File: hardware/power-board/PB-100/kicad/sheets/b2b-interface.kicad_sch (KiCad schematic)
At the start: 1 part

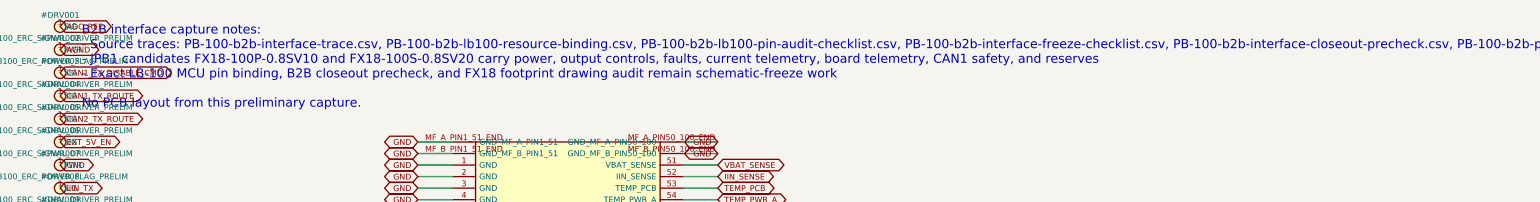
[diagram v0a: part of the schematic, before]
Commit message: feat(hardware): close LB FB schematics and FX18 mechanics
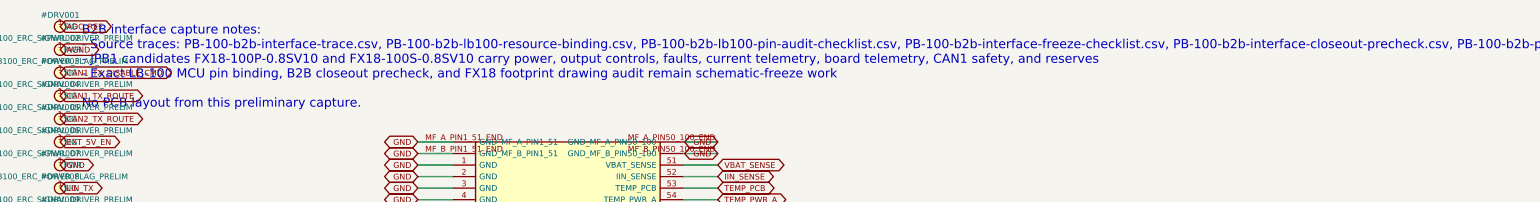
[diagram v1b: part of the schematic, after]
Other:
- note added: "B2B interface capture notes: - Source traces: PB-100-b2b-interface-trace.csv, PB-100-b2b-lb100-resource-binding.csv, PB-100-b2b-lb100-pin-audit-checklist.csv, PB-100-b2b-interface-freeze-checklist.csv, PB-100-b2b-interface-closeout-precheck.csv, PB-100-b2b-pin-map.csv, PB-100-b2b-pin-budget.csv - JPB1 candidates FX18-100P-0.8SV10 and FX18-100S-0.8SV10 carry power, output controls, faults, current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"
- note removed: "B2B interface capture notes: - Source traces: PB-100-b2b-interface-trace.csv, PB-100-b2b-lb100-resource-binding.csv, PB-100-b2b-lb100-pin-audit-checklist.csv, PB-100-b2b-interface-freeze-checklist.csv, PB-100-b2b-interface-closeout-precheck.csv, PB-100-b2b-pin-map.csv, PB-100-b2b-pin-budget.csv - JPB1 candidates FX18-100P-0.8SV10 and FX18-100S-0.8SV20 carry power, output controls, faults, current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"
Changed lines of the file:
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@@
     (comment 2 "Sources: PB-100-b2b-interface-trace.csv, PB-100-b2b-lb100-resource-binding.csv, PB-100-b2b-lb100-pin-audit-checklist.csv, PB-100-b2b-interface-freeze-checklist.csv, PB-100-b2b-interface-closeout-precheck.csv, and PB-100-b2b-pin-map.csv.")
   )
-  (text "B2B interface capture notes:\n- Source traces: PB-100-b2b-interface-trace.csv, PB-100-b2b-lb100-resource-binding.csv, PB-100-b2b-lb100-pin-audit-checklist.csv, PB-100-b2b-interface-freeze-checklist.csv, PB-100-b2b-interface-closeout-precheck.csv, PB-100-b2b-pin-map.csv, PB-100-b2b-pin-budget.csv\n- JPB1 candidates FX18-100P-0.8SV10 and FX18-100S-0.8SV20 carry power, output controls, faults, current telemetry, board telemetry, CAN1 safety, and reserves\n- Exact LB-100 MCU pin binding, B2B closeout precheck, and FX18 footprint drawing audit remain schematic-freeze work\n\nNo PCB layout from this preliminary capture."
+  (text "B2B interface capture notes:\n- Source traces: PB-100-b2b-interface-trace.csv, PB-100-b2b-lb100-resource-binding.csv, PB-100-b2b-lb100-pin-audit-checklist.csv, PB-100-b2b-interface-freeze-checklist.csv, PB-100-b2b-interface-closeout-precheck.csv, PB-100-b2b-pin-map.csv, PB-100-b2b-pin-budget.csv\n- JPB1 candidates FX18-100P-0.8SV10 and FX18-100S-0.8SV10 carry power, output controls, faults, current telemetry, board telemetry, CAN1 safety, and reserves\n- Exact LB-100 MCU pin binding, B2B closeout precheck, and FX18 footprint drawing audit remain schematic-freeze work\n\nNo PCB layout from this preliminary capture."
     (at 20 20 0)
     (effects (font (size 2.0 2.0)) (justify left top))
